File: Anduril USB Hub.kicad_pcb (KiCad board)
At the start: 4 copper layers, 80.4 x 80.6 mm, 38 parts, among them J1 USB C 2.0, Upstream, J2 USB A, Port 1, J3 USB C 2.0, Port 2, J4 USB A, Port 3, U1 USB4604-1080HN, U2 USBLC6-2SC6, U3 USBLC6-2SC6, U4 USBLC6-2SC6, Y1 24M

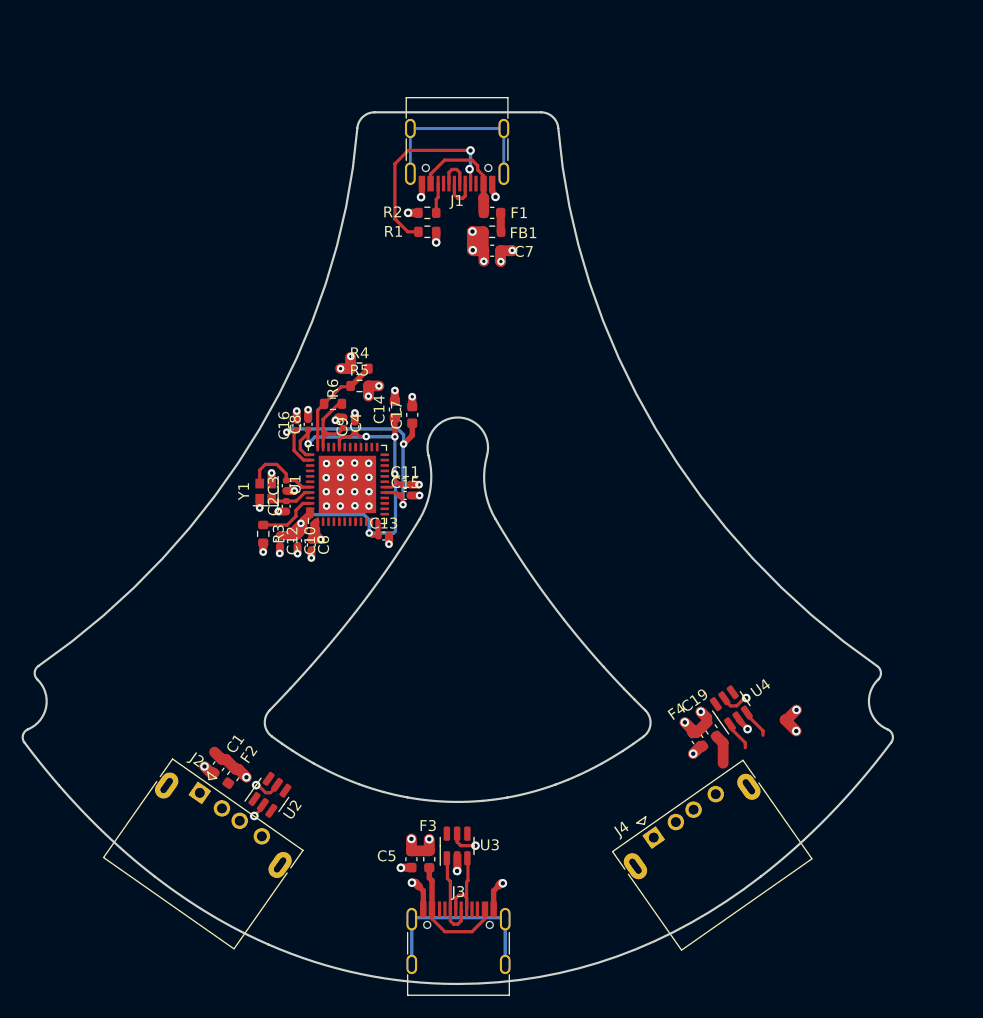
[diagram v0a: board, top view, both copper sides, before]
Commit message: V1.0
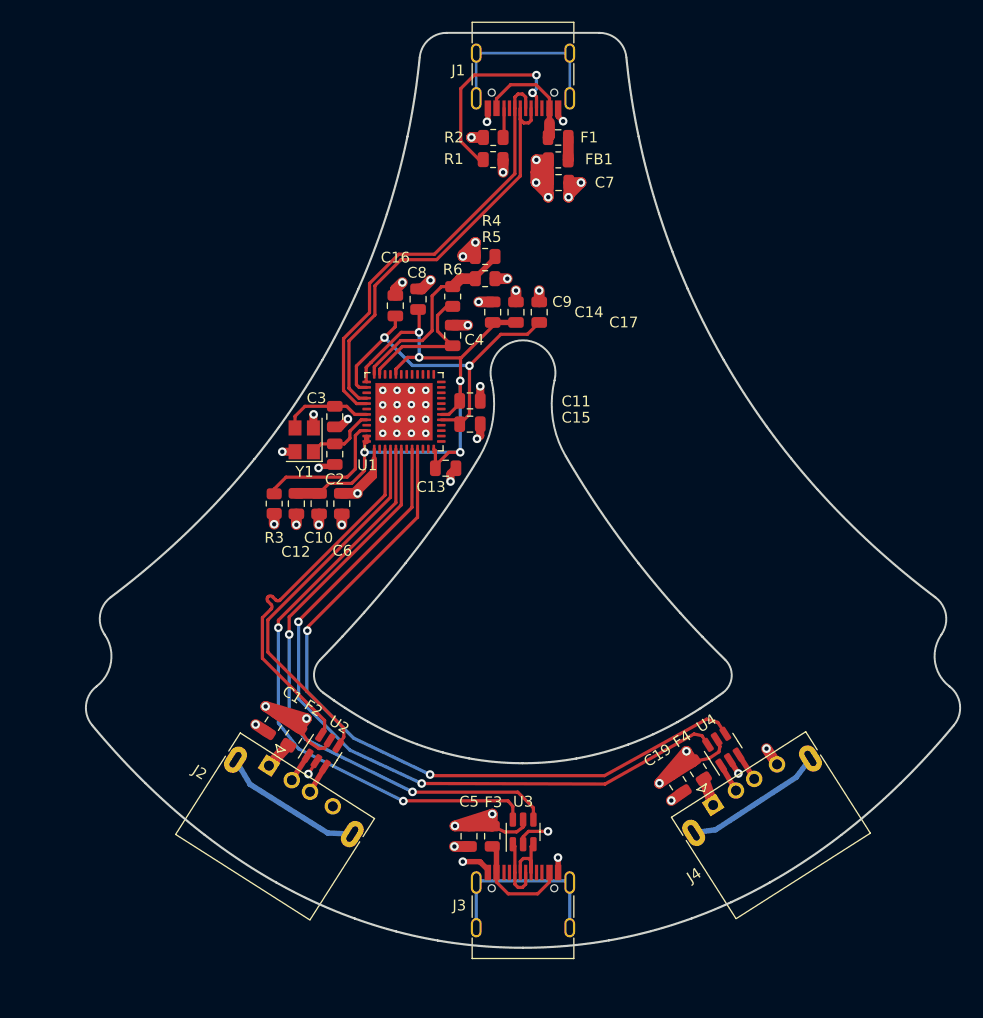
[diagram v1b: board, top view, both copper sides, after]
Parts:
- C1, C14, C17, C19, C5, C7: footprint Capacitor_SMD:C_0603_1608Metric -> Capacitor_SMD:C_0805_2012Metric
- C10, C11, C12, C13, C15, C16, C2, C3, C4, C6, C8, C9: footprint Capacitor_SMD:C_0402_1005Metric -> Capacitor_SMD:C_0805_2012Metric
- F1, F2, F3, F4: footprint Fuse:Fuse_0603_1608Metric -> Fuse:Fuse_0805_2012Metric
- FB1, R1, R2, R3, R4, R5, R6: footprint Resistor_SMD:R_0603_1608Metric -> Resistor_SMD:R_0805_2012Metric
- Y1: footprint Crystal:Crystal_SMD_2016-4Pin_2.0x1.6mm -> Crystal:Crystal_SMD_3225-4Pin_3.2x2.5mm
- moved C9 16.6 mm to (109.6, 56.6)
- moved R4 15.6 mm to (108.9, 51.4)
- moved C8 15.4 mm to (102.7, 55.4)
- moved R5 15.3 mm to (108.9, 53.5)
- moved C17 15.1 mm to (113.9, 56.6)
- moved R6 14.9 mm to (105.9, 55.1), turned to -90 degrees
- moved C14 14.4 mm to (111.7, 56.6)
- moved C16 14.3 mm to (100.6, 56.0)
- moved C4 12.9 mm to (105.9, 58.7)
- moved C11 9.79 mm to (107.5, 64.8)
- moved F1 9.26 mm to (115.6, 40.4)
- moved J1 9.26 mm to (112.4, 33.7)
- moved R2 9.26 mm to (109.6, 40.4)
- moved R1 9.03 mm to (109.6, 42.5)
- moved FB1 9.03 mm to (115.7, 42.5)
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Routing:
- net P3 D+: track 0.00 -> 69.9 mm, vias 0 -> 2
- net P3 D-: track 0.00 -> 69.6 mm, vias 0 -> 2
- net P2 D+: track 0.00 -> 55.5 mm, vias 0 -> 2
- net P2 D-: track 0.00 -> 55.3 mm, vias 0 -> 2
- net UP D+: track 3.28 -> 40.5 mm
- net UP D-: track 3.39 -> 39.8 mm
- net P1 D+: track 0.00 -> 35.2 mm
- net P1 D-: track 0.00 -> 35.1 mm
- net +5V: track 35.2 -> 68.6 mm, vias 14 -> 12
- net unconnected-(J2-Pad5): track 0.00 -> 13.4 mm
- net unconnected-(J4-Pad5): track 0.00 -> 13.1 mm
- net VDD33: track 50.5 -> 62.7 mm, vias 6 -> 5
- net GND: track 39.3 -> 48.2 mm, vias 51 -> 49
- net +3V3: track 10.00 -> 18.1 mm
- net Net-(R3-Pad1): track 5.48 -> 13.0 mm
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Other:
- board size 80.4 x 80.6 mm -> 80.8 x 84.6 mm
- rule pad_to_mask_clearance: 0.05 -> 0
- board text added: ":D designs Anduril USB Hub v1.0 Dec 2022"
- board text added: "To the amazing employees of Anduril Industries Dec 2022"
- board text added: "USB 2.0 1A Input Fuse 900mA Output Fuse per port"
